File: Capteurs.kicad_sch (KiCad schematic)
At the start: 5 parts, among them U1 BME280

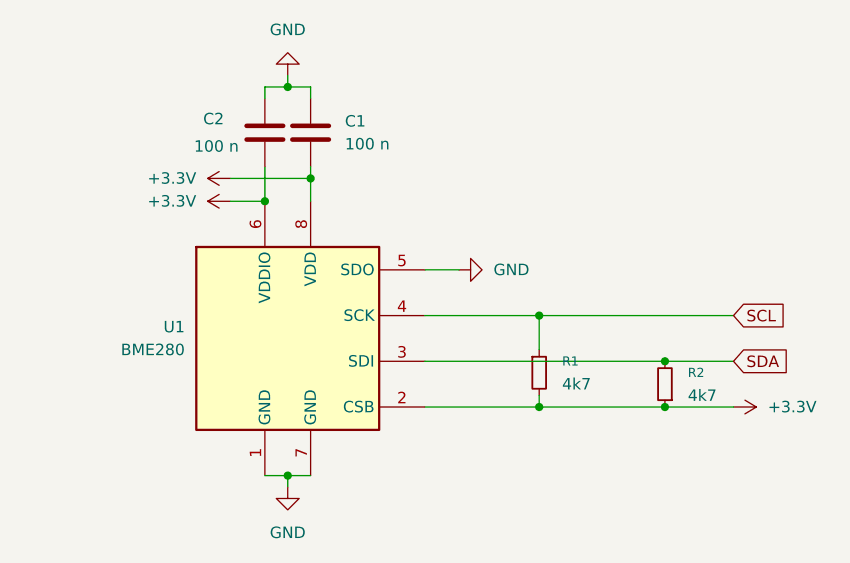
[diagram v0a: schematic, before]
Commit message: schema v1
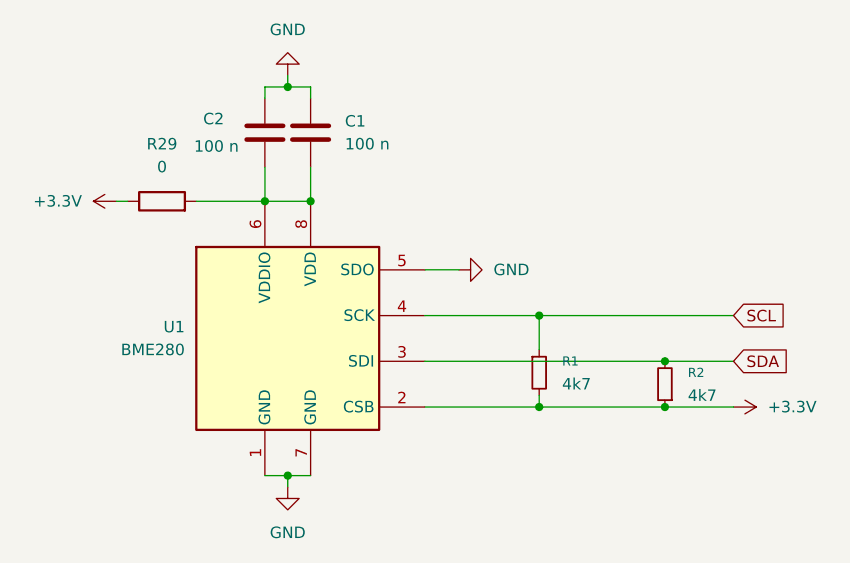
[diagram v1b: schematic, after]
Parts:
- added R29: 0, symbol Device:R
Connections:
- net +3.3V: now also R29.1; no longer C1.1, C2.2, U1.6 (VDDIO), U1.8 (VDD)
- new net: C1.1, C2.2, R29.2, U1.6 (VDDIO), U1.8 (VDD)
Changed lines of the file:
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@@
-	)
-	(junction
-		(at 142.24 74.93)
-		(diameter 0)
-		(color 0 0 0 0)
 	)
 	(junction
@@
 	)
 	(junction
+		(at 142.24 77.47)
+		(diameter 0)
+		(color 0 0 0 0)
+	)
+	(junction
 		(at 181.61 100.33)
 		(diameter 0)
@@
 	(wire
 		(pts
-			(xy 133.35 77.47) (xy 137.16 77.47)
-		)
-		(stroke
-			(width 0)
-			(type default)
-		)
-	)
-	(wire
-		(pts
-			(xy 133.35 74.93) (xy 142.24 74.93)
-		)
-		(stroke
-			(width 0)
-			(type default)
-		)
-	)
-	(wire
-		(pts
 			(xy 181.61 95.25) (xy 189.23 95.25)
 		)
@@
 	(wire
 		(pts
+			(xy 129.54 77.47) (xy 137.16 77.47)
+		)
+		(stroke
+			(width 0)
+			(type default)
+		)
+	)
+	(wire
+		(pts
 			(xy 167.64 99.06) (xy 167.64 100.33)
 		)
@@
 	(wire
 		(pts
-			(xy 142.24 73.66) (xy 142.24 74.93)
-		)
-		(stroke
-			(width 0)
-			(type default)
-		)
-	)
-	(wire
-		(pts
 			(xy 142.24 64.77) (xy 142.24 66.04)
 		)
@@
 	(wire
 		(pts
-			(xy 142.24 74.93) (xy 142.24 77.47)
+			(xy 142.24 73.66) (xy 142.24 77.47)
 		)
 		(stroke
@@
 		(pts
 			(xy 154.94 85.09) (xy 158.75 85.09)
+		)
+		(stroke
+			(width 0)
+			(type default)
+		)
+	)
+	(wire
+		(pts
+			(xy 120.65 77.47) (xy 121.92 77.47)
+		)
+		(stroke
+			(width 0)
+			(type default)
+		)
+	)
+	(wire
+		(pts
+			(xy 137.16 77.47) (xy 142.24 77.47)
 		)
 		(stroke
@@
 				(justify left)
 				(hide yes)
+			)
+		)
+	)
+	(symbol
+		(lib_id "Device:R")
+		(at 125.73 77.47 90)
+		(unit 1)
+		(exclude_from_sim no)
+		(in_bom yes)
+		(on_board yes)
+		(dnp no)
+		(fields_autoplaced yes)
+		(property "Reference" "R29"
+			(at 125.73 71.12 90)
+			(effects
+				(font
+					(size 1.27 1.27)
+				)
+			)
+		)
+		(property "Value" "0"
+			(at 125.73 73.66 90)
+			(effects
+				(font
+					(size 1.27 1.27)
+				)
+			)
+		)
+		(property "Footprint" ""
+			(at 125.73 79.248 90)
+			(effects
+				(font
+					(size 1.27 1.27)
+				)
+				(hide yes)
+			)
+		)
+		(property "Datasheet" "~"
+			(at 125.73 77.47 0)
+			(effects
+				(font
+					(size 1.27 1.27)
+				)
+				(hide yes)
+			)
+		)
+		(property "Description" "Resistor"
+			(at 125.73 77.47 0)
+			(effects
+				(font
+					(size 1.27 1.27)
+				)
+				(hide yes)
+			)
+		)
+		(property "LCSC" "C21189"
+			(at 125.73 77.47 0)
+			(effects
+				(font
+					(size 1.27 1.27)
+				)
+				(hide yes)
+			)
+		)
+		(pin "1"
+		)
+		(pin "2"
+		)
+		(instances
+			(project "Station_Meteo_pcb"
+				(path "/90bd0b60-6e70-43e1-8410-99fb54688c17/d62bceb2-9908-4d7c-aad2-bbefb30f6285"
+					(reference "R29")
+					(unit 1)
+				)
 			)
 		)
@@
 	(symbol
 		(lib_id "power:+3.3V")
-		(at 133.35 77.47 90)
+		(at 120.65 77.47 90)
 		(unit 1)
 		(exclude_from_sim no)
@@
 		(dnp no)
 		(property "Reference" "#PWR02"
-			(at 137.16 77.47 0)
+			(at 124.46 77.47 0)
 			(effects
 				(font
@@
 		)
 		(property "Value" "+3.3V"
-			(at 129.54 77.4701 90)
+			(at 116.84 77.4701 90)
 			(effects
 				(font
@@
 		)
 		(property "Footprint" ""
-			(at 133.35 77.47 0)
+			(at 120.65 77.47 0)
 			(effects
 				(font
@@
 		)
 		(property "Datasheet" ""
-			(at 133.35 77.47 0)
+			(at 120.65 77.47 0)
 			(effects
 				(font
@@
 		)
 		(property "Description" "Power symbol creates a global label with name \"+3.3V\""
-			(at 133.35 77.47 0)
+			(at 120.65 77.47 0)
 			(effects
 				(font
@@
 					(unit 1)
 				)
-			)
-		)
-	)
-	(symbol
-		(lib_id "power:+3.3V")
-		(at 133.35 74.93 90)
-		(unit 1)
-		(exclude_from_sim no)
-		(in_bom yes)
-		(on_board yes)
-		(dnp no)
-		(property "Reference" "#PWR03"
-			(at 137.16 74.93 0)
-			(effects
-				(font
-					(size 1.27 1.27)
-				)
-				(hide yes)
-			)
-		)
-		(property "Value" "+3.3V"
-			(at 129.54 74.9301 90)
-			(effects
-				(font
-					(size 1.27 1.27)
-				)
-				(justify left)
-			)
-		)
-		(property "Footprint" ""
-			(at 133.35 74.93 0)
-			(effects
-				(font
-					(size 1.27 1.27)
-				)
-				(hide yes)
-			)
-		)
-		(property "Datasheet" ""
-			(at 133.35 74.93 0)
-			(effects
-				(font
-					(size 1.27 1.27)
-				)
-				(hide yes)
-			)
-		)
-		(property "Description" "Power symbol creates a global label with name \"+3.3V\""
-			(at 133.35 74.93 0)
-			(effects
-				(font
-					(size 1.27 1.27)
-				)
-				(hide yes)
-			)
-		)
-		(pin "1"
-		)
-		(instances
-			(project "Station_Meteo_pcb"
-				(path "/90bd0b60-6e70-43e1-8410-99fb54688c17/d62bceb2-9908-4d7c-aad2-bbefb30f6285"
-					(reference "#PWR03")
-					(unit 1)
-				)
